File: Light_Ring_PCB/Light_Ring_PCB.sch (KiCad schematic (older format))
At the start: 126 parts, among them J1 LIGHT_OUT, Q1 Q_Photo_NPN, Q10 Q_Photo_NPN, Q11 Q_Photo_NPN, Q12 Q_Photo_NPN, Q13 Q_Photo_NPN, Q14 Q_Photo_NPN, Q15 Q_Photo_NPN, Q16 Q_Photo_NPN, Q17 Q_Photo_NPN, Q18 Q_Photo_NPN, Q19 Q_Photo_NPN, Q2 Q_Photo_NPN, Q20 Q_Photo_NPN, Q21 Q_Photo_NPN, Q22 Q_Photo_NPN, Q23 Q_Photo_NPN, Q24 Q_Photo_NPN, Q25 EN, Q3 Q_Photo_NPN, Q4 Q_Photo_NPN, Q5 Q_Photo_NPN, Q6 Q_Photo_NPN, Q7 Q_Photo_NPN, Q8 Q_Photo_NPN, Q9 Q_Photo_NPN, U1 ADG732

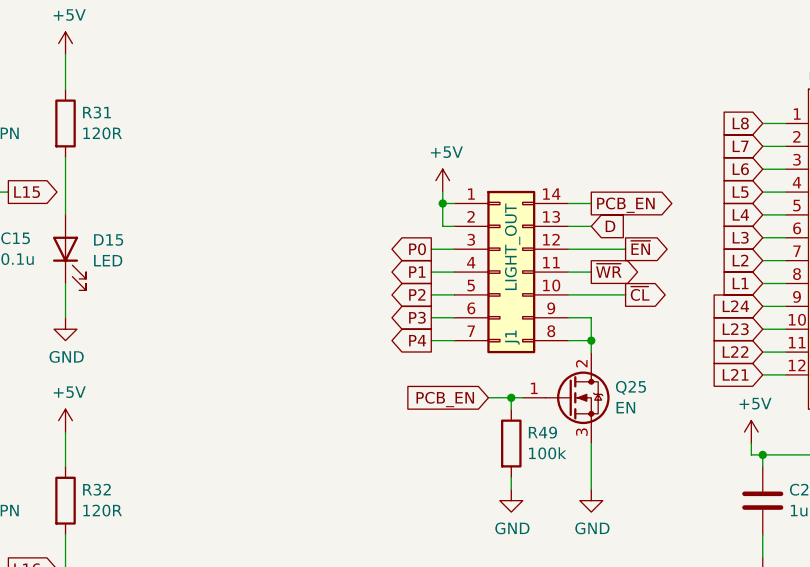
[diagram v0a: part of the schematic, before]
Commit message: Finalizing Main PCB Sch
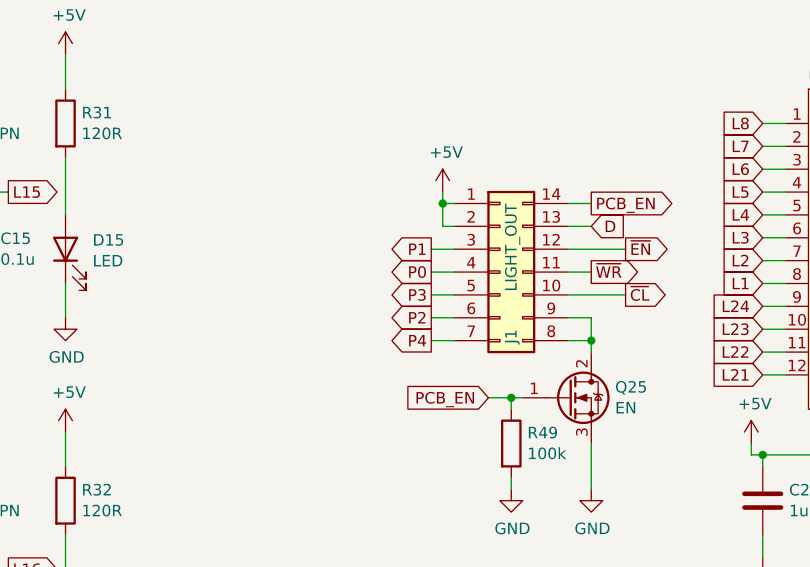
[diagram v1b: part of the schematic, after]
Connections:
- net P0: now also J1.4 (Pin_4); no longer J1.3 (Pin_3)
- net P1: now also J1.3 (Pin_3); no longer J1.4 (Pin_4)
- net P2: now also J1.6 (Pin_6); no longer J1.5 (Pin_5)
- net P3: now also J1.5 (Pin_5); no longer J1.6 (Pin_6)
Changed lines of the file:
@@
 Wire Wire Line
 	7350 5050 7600 5050
+Text GLabel 6750 4950 0    50   Output ~ 0
+P0
 Text GLabel 6750 4850 0    50   Output ~ 0
-P0
-Text GLabel 6750 4950 0    50   Output ~ 0
 P1
+Text GLabel 6750 5150 0    50   Output ~ 0
+P2
 Text GLabel 6750 5050 0    50   Output ~ 0
-P2
-Text GLabel 6750 5150 0    50   Output ~ 0
 P3
 Text GLabel 6750 5250 0    50   Output ~ 0
 P4
-Wire Wire Line
-	6750 4850 6850 4850
-Wire Wire Line
-	6750 4950 6850 4950
 Wire Wire Line
 	6750 5050 6850 5050
@@
 Wire Wire Line
 	10200 5400 10100 5400
+Wire Wire Line
+	6750 4950 6850 4950
+Wire Wire Line
+	6750 4850 6850 4850
 $EndSCHEMATC
